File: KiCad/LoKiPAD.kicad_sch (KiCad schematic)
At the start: 57 parts, among them J1 AudioJack4, J2 Conn_01x07_Female, J3 AudioJack4, SW1 SW_Push, SW10 SW_Push, SW11 SW_Push, SW12 SW_Push, SW13 Rotary_Encoder_Switch, SW2 SW_Push, SW3 SW_Push, SW4 SW_Push, SW5 SW_Push, SW6 SW_Push, SW7 SW_Push, SW8 SW_Push, SW9 SW_Push, U1 Pico, U2 H11L1

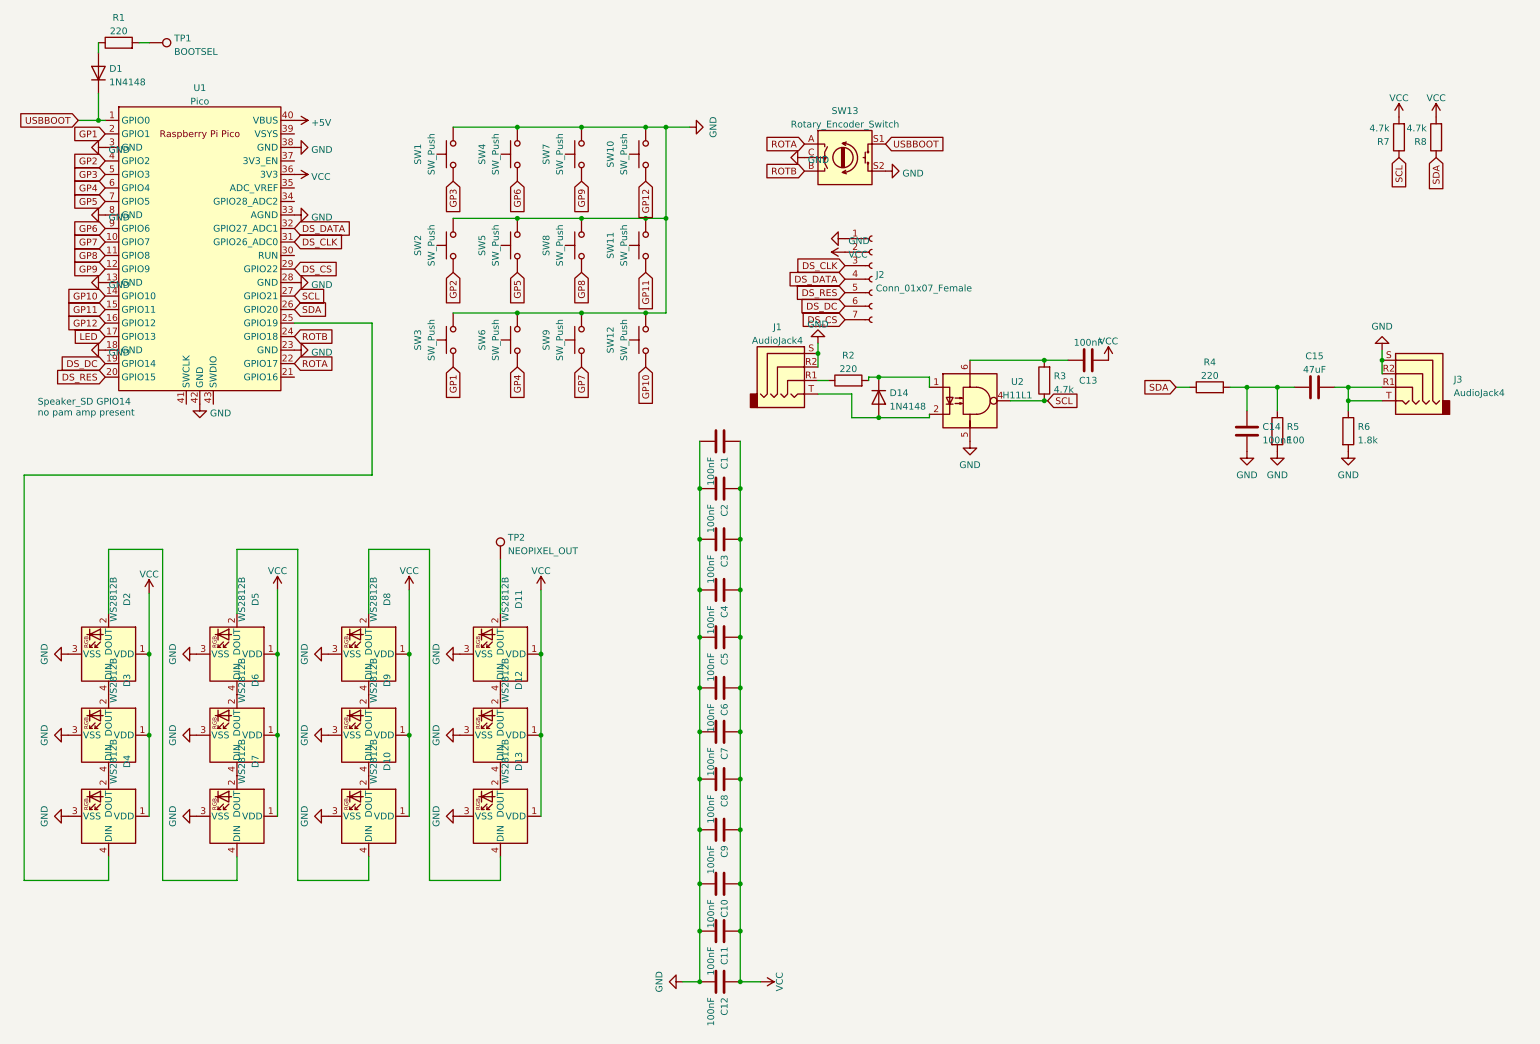
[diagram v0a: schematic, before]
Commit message: more parts moved to back, kicad7
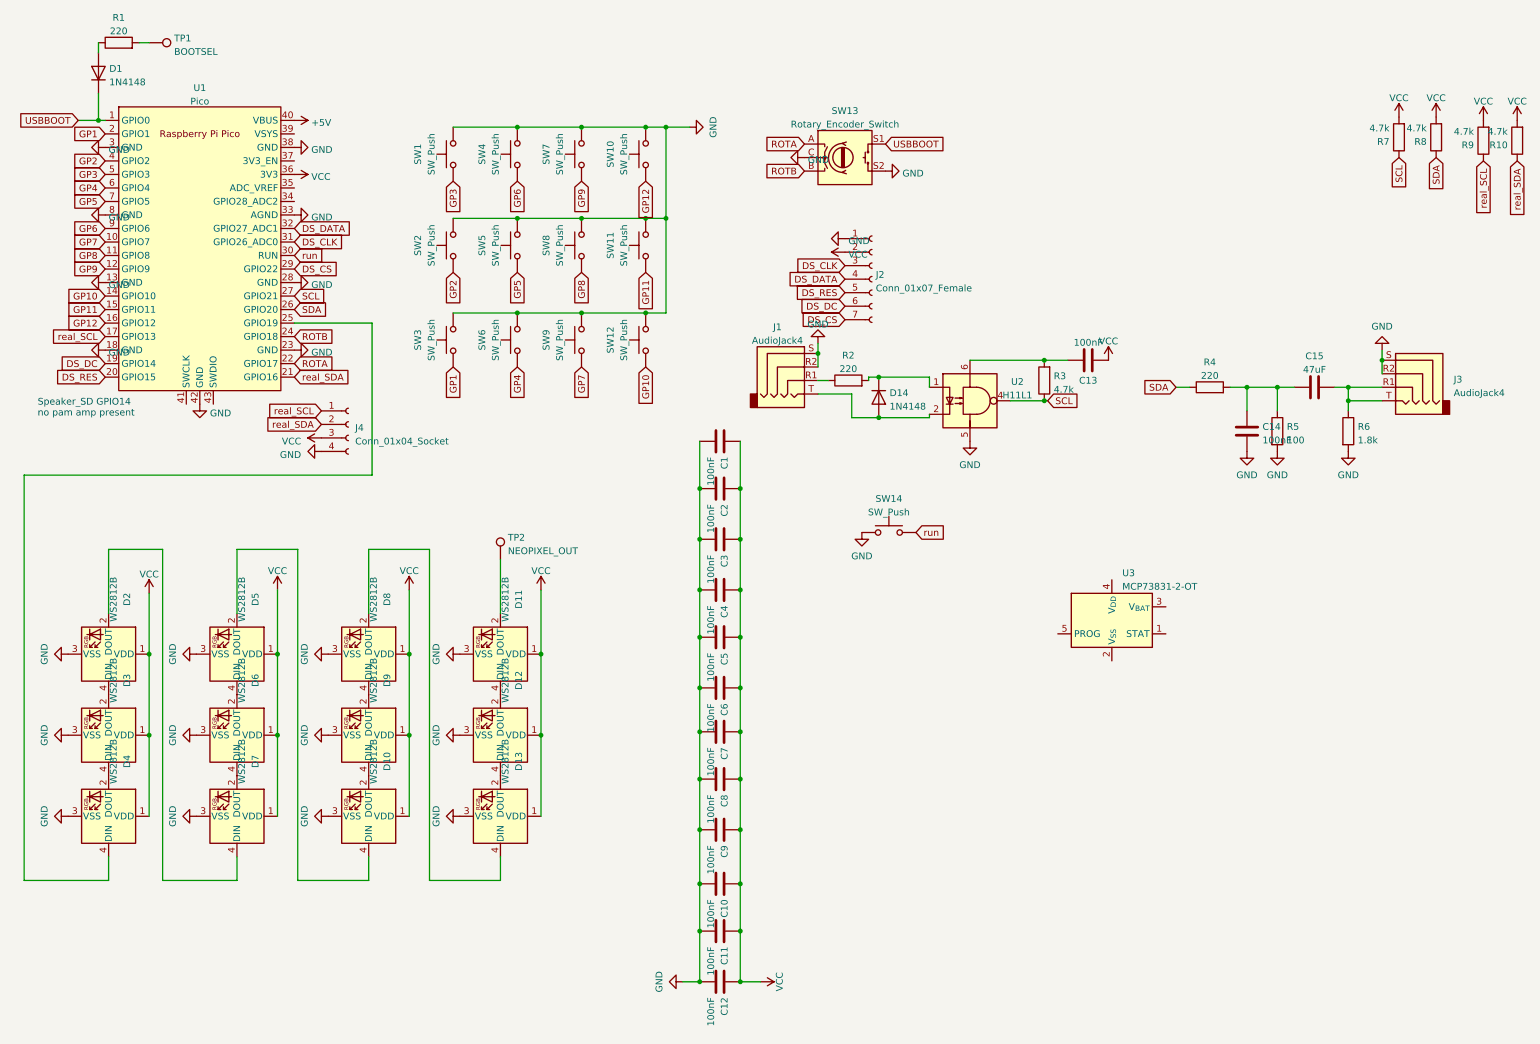
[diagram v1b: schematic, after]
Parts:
- added J4: Conn_01x04_Socket, Connector_JST:JST_SH_BM04B-SRSS-TB_1x04-1MP_P1.00mm_Vertical, symbol Connector:Conn_01x04_Socket
- added R10, R9: 4.7k, Resistor_SMD:R_0603_1608Metric_Pad0.98x0.95mm_HandSolder, symbol Device:R
- added SW14: SW_Push, Button_Switch_SMD:SW_Push_1P1T_NO_CK_KMR2, symbol Switch:SW_Push
- added U3: MCP73831-2-OT, Package_TO_SOT_SMD:SOT-23-5, symbol Battery_Management:MCP73831-2-OT
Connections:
- net GND: now also J4.4 (Pin_4), SW14.1
- net VCC: now also J4.3 (Pin_3), R10.2, R9.2
- net real_SDA: now reaches U1.21 (GPIO16)
- net real_SDA: now also J4.2 (Pin_2), R10.1
- net run: now reaches U1.30 (RUN)
- net run: now also SW14.2
- net LED renamed real_SCL
- net real_SCL: now also J4.1 (Pin_1), R9.1
